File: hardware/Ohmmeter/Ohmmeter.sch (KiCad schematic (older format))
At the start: 52 parts, among them Q1 KT361, Q10 KT361, Q11 KT361, Q2 KT361, Q3 KT361, Q4 KT361, Q5 KT361, Q6 KT361, Q7 KT361, Q8 KT361, Q9 KT361, U1 L78L05_TO92, U2 LP2950-3.3_TO92, U3 ATmega8A-PU

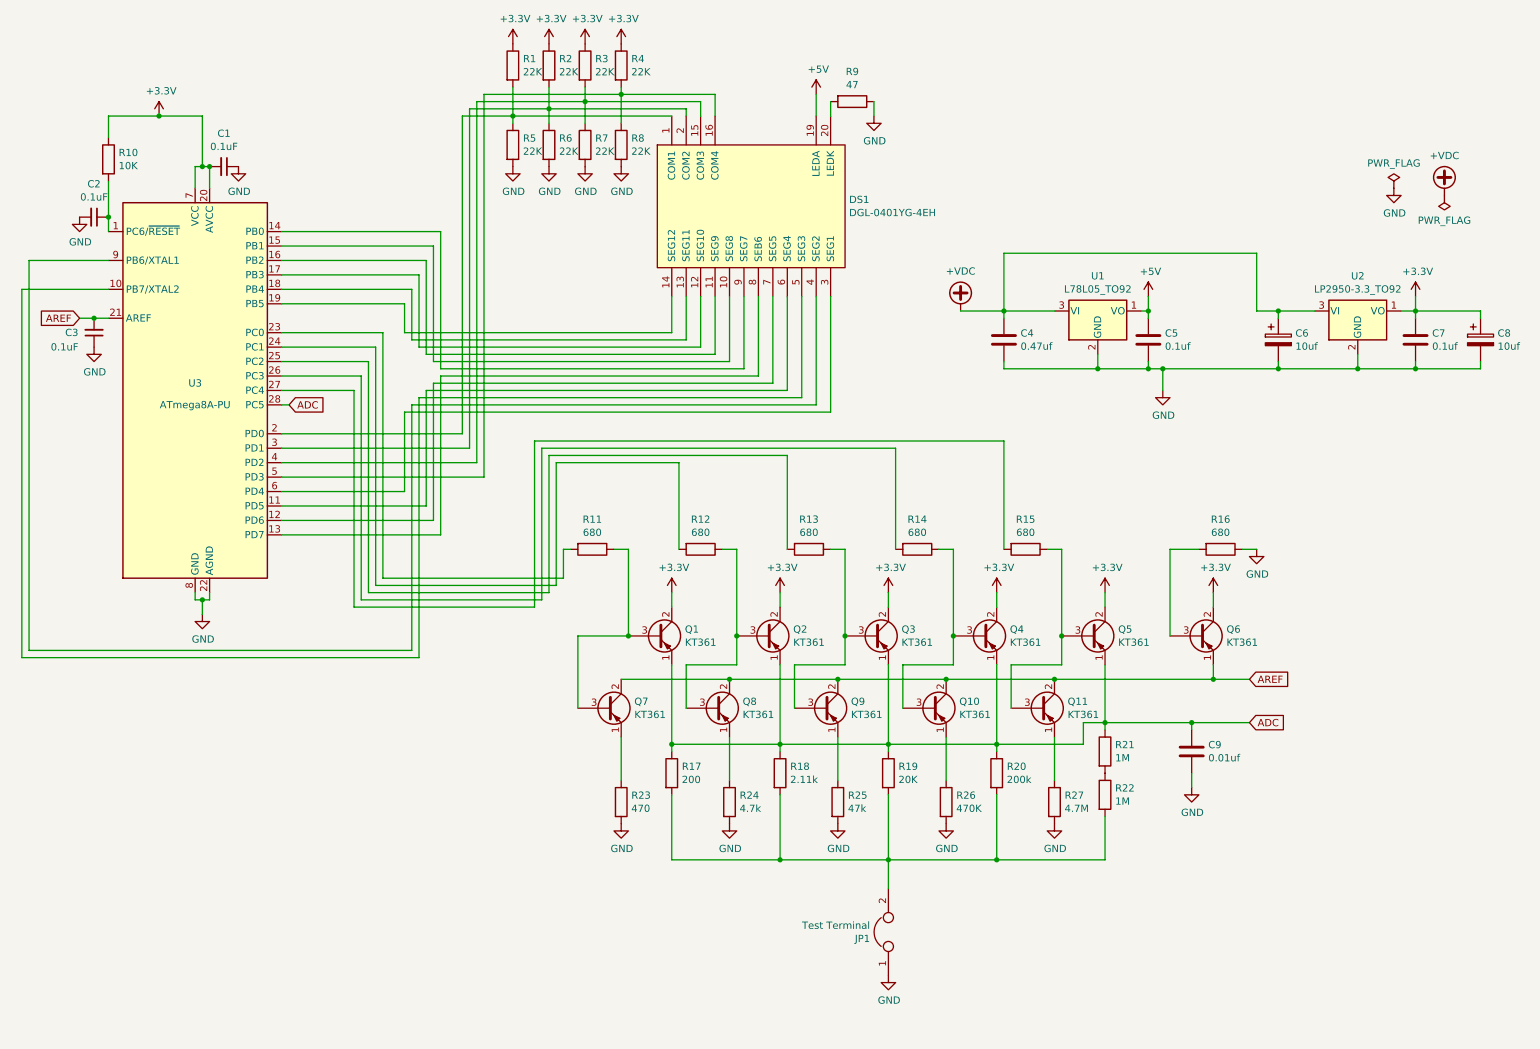
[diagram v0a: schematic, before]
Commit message: Hardware updates. Changed the algorithm to use fewer lookup tables.
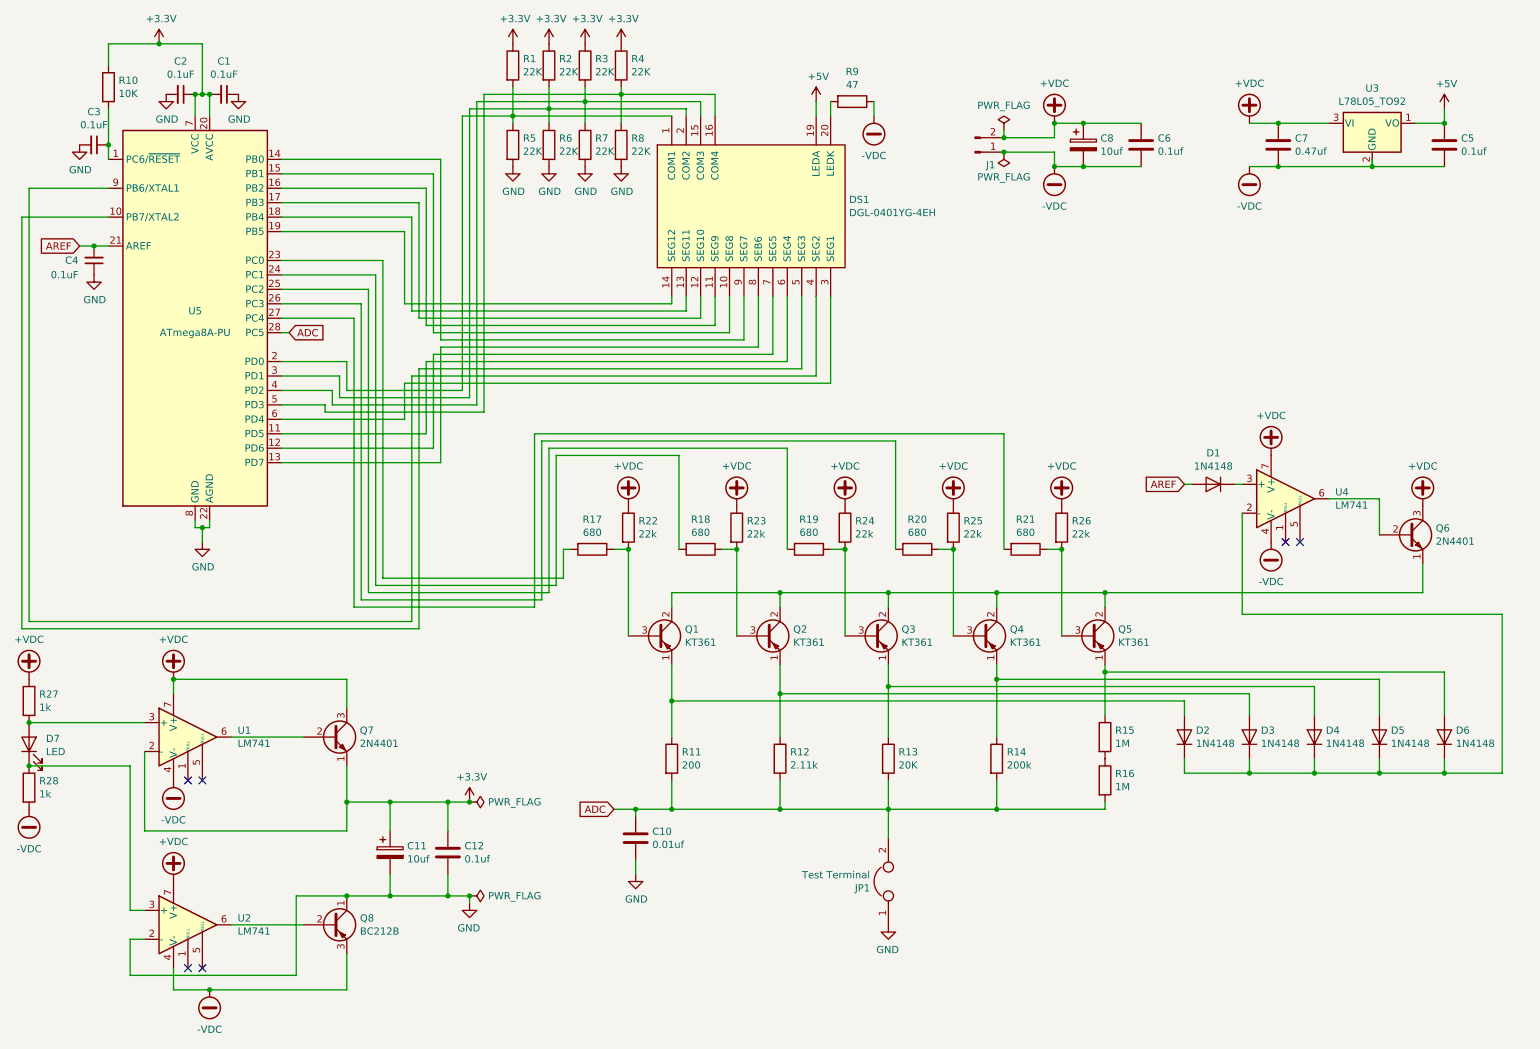
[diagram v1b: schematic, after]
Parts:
- removed C7: 0.1uf, symbol Device:C
- removed C8: 10uf, symbol Device:CP
- removed Q10, Q11, Q6, Q7, Q8, Q9: KT361, symbol Device:Q_PNP_ECB
- removed R16: 680, symbol Device:R
- removed U2: LP2950-3.3_TO92, Package_TO_SOT_THT:TO-92_Inline, symbol Regulator_Linear:LP2950-3.3_TO92
- added C11: 10uf, Capacitor_THT:CP_Radial_D6.3mm_P2.50mm, symbol Device:CP
- added C12, C6: 0.1uf, Resistor_THT:R_Axial_DIN0309_L9.0mm_D3.2mm_P2.54mm_Vertical, symbol Device:C
- added C2: 0.1uF, Resistor_THT:R_Axial_DIN0309_L9.0mm_D3.2mm_P2.54mm_Vertical, symbol Device:C_Small
- added D1, D2, D3, D4, D5, D6: 1N4148, Diode_THT:D_DO-35_SOD27_P7.62mm_Horizontal, symbol Device:D
- added D7: LED, LED_THT:LED_D10.0mm, symbol Device:LED
- added J1: Power, Connector_PinHeader_2.54mm:PinHeader_1x02_P2.54mm_Horizontal, symbol Connector:Conn_01x02_Male
- added Q6, Q7: 2N4401, Package_TO_SOT_THT:TO-92_Inline_Wide, symbol Device:Q_NPN_EBC
- added Q8: BC212B, Package_TO_SOT_THT:TO-92_Inline_Wide, symbol Device:Q_PNP_CBE
- added R22: 22k, Resistor_THT:R_Axial_DIN0207_L6.3mm_D2.5mm_P7.62mm_Horizontal, symbol Device:R
- added R28: 1k, Resistor_THT:R_Axial_DIN0207_L6.3mm_D2.5mm_P7.62mm_Horizontal, symbol Device:R
- added U1, U2, U4: LM741, Package_DIP:DIP-8_W7.62mm_Socket, symbol Amplifier_Operational:LM741
- C1, C5: footprint (none) -> Resistor_THT:R_Axial_DIN0309_L9.0mm_D3.2mm_P2.54mm_Vertical
- C10: renamed from C9; footprint (none) -> Capacitor_THT:C_Rect_L7.0mm_W2.0mm_P5.00mm
- C3: renamed from C2; footprint (none) -> Resistor_THT:R_Axial_DIN0309_L9.0mm_D3.2mm_P2.54mm_Vertical
- C4: renamed from C3; footprint (none) -> Resistor_THT:R_Axial_DIN0309_L9.0mm_D3.2mm_P2.54mm_Vertical
- C7: renamed from C4; footprint (none) -> Capacitor_THT:C_Rect_L7.0mm_W4.5mm_P5.00mm
- C8: renamed from C6; footprint (none) -> Capacitor_THT:CP_Radial_D6.3mm_P2.50mm
- DS1: footprint (none) -> Connector_PinHeader_2.54mm:PinHeader_1x20_P2.54mm_Horizontal
- JP1: footprint (none) -> Connector_PinHeader_2.54mm:PinHeader_1x02_P2.54mm_Horizontal
- Q1, Q2, Q3, Q4, Q5: footprint (none) -> JRMKiCadLibrary:KT-13
- R1, R10, R2, R3, R4, R5, R6, R7, R8, R9: footprint (none) -> Resistor_THT:R_Axial_DIN0207_L6.3mm_D2.5mm_P7.62mm_Horizontal
- R11: renamed from R17; footprint (none) -> Resistor_THT:R_Axial_DIN0207_L6.3mm_D2.5mm_P10.16mm_Horizontal
- R12: renamed from R18; footprint (none) -> Resistor_THT:R_Axial_DIN0207_L6.3mm_D2.5mm_P10.16mm_Horizontal
- R13: renamed from R19; footprint (none) -> Resistor_THT:R_Axial_DIN0207_L6.3mm_D2.5mm_P10.16mm_Horizontal
- R14: renamed from R20; footprint (none) -> Resistor_THT:R_Axial_DIN0207_L6.3mm_D2.5mm_P10.16mm_Horizontal
- R15: renamed from R21; footprint (none) -> Resistor_THT:R_Axial_DIN0614_L14.3mm_D5.7mm_P5.08mm_Vertical
- R16: renamed from R22; footprint (none) -> Resistor_THT:R_Axial_DIN0614_L14.3mm_D5.7mm_P5.08mm_Vertical
- R17: renamed from R11; footprint (none) -> Resistor_THT:R_Axial_DIN0207_L6.3mm_D2.5mm_P7.62mm_Horizontal
- R18: renamed from R12; footprint (none) -> Resistor_THT:R_Axial_DIN0207_L6.3mm_D2.5mm_P7.62mm_Horizontal
- R19: renamed from R13; footprint (none) -> Resistor_THT:R_Axial_DIN0207_L6.3mm_D2.5mm_P7.62mm_Horizontal
- R20: renamed from R14; footprint (none) -> Resistor_THT:R_Axial_DIN0207_L6.3mm_D2.5mm_P7.62mm_Horizontal
- R21: renamed from R15; footprint (none) -> Resistor_THT:R_Axial_DIN0207_L6.3mm_D2.5mm_P7.62mm_Horizontal
- R23: value 470 -> 22k; footprint (none) -> Resistor_THT:R_Axial_DIN0207_L6.3mm_D2.5mm_P7.62mm_Horizontal
- R24: value 4.7k -> 22k; footprint (none) -> Resistor_THT:R_Axial_DIN0207_L6.3mm_D2.5mm_P7.62mm_Horizontal
- R25: value 47k -> 22k; footprint (none) -> Resistor_THT:R_Axial_DIN0207_L6.3mm_D2.5mm_P7.62mm_Horizontal
- R26: value 470K -> 22k; footprint (none) -> Resistor_THT:R_Axial_DIN0207_L6.3mm_D2.5mm_P7.62mm_Horizontal
- R27: value 4.7M -> 1k; footprint (none) -> Resistor_THT:R_Axial_DIN0207_L6.3mm_D2.5mm_P7.62mm_Horizontal
- U3: renamed from U1; footprint Package_TO_SOT_THT:TO-92_Inline -> Package_TO_SOT_THT:TO-92_Inline_Wide
- U5: renamed from U3; footprint Package_DIP:DIP-28_W7.62mm -> Package_DIP:DIP-28_W7.62mm_Socket
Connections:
- net +3V3: now also C11.1, C12.1, C2.1, Q7.1 (E), U1.2 (-); no longer Q1.2 (C), Q2.2 (C), Q3.2 (C), Q4.2 (C), Q5.2 (C)
- net +VDC: now also R23.1, R24.1, R25.1, R26.1, R27.1, C6.1, J1.2 (Pin_2), Q6.3 (C), Q7.3 (C), R22.1, U1.7 (V+), U2.7 (V+), U4.7 (V+)
- net ADC: now also JP1.2, R11.2, R12.2, R13.2, R14.2, R16.2; no longer Q1.1 (E), Q2.1 (E), Q3.1 (E), Q4.1 (E), Q5.1 (E), R11.1, R12.1, R13.1, R14.1, R15.1
- net AREF: now also D1.2 (A)
- net GND: now also C11.2, C12.2, C2.2, Q8.1 (C), U2.2 (-); no longer C5.2, C7.2, C8.2, R23.2, R24.2, R25.2, R26.2, R27.2, R9.1, U3.2 (GND)
- net at Q5.3 (B), R21.1: now also R26.2
- net at Q2.3 (B), R18.1: now also R23.2
- net at Q3.3 (B), R19.1: now also R24.2
- net at Q4.3 (B), R20.1: now also R25.2
- net at Q1.3 (B), R17.1: now also R22.2
- net at DS1.15 (NC): now also R3.2, R7.1, U5.4 (PD2)
- net at DS1.16 (NC): now also R4.2, R8.1, U5.5 (PD3)
- new net: D6.2 (A), Q5.1 (E), R15.1
- new net: Q1.2 (C), Q2.2 (C), Q3.2 (C), Q4.2 (C), Q5.2 (C), Q6.1 (E)
- new net: D3.2 (A), Q2.1 (E), R12.1
- new net: D4.2 (A), Q3.1 (E), R13.1
- new net: D5.2 (A), Q4.1 (E), R14.1
- new net: D2.2 (A), Q1.1 (E), R11.1
- new net: D7.1 (K), R28.1, U2.3 (+)
- new net: D7.2 (A), R27.2, U1.3 (+)
- new net: Q7.2 (B), U1.6
- new net: Q8.2 (B), U2.6
- new net: Q6.2 (B), U4.6
- new net: D2.1 (K), D3.1 (K), D4.1 (K), D5.1 (K), D6.1 (K), U4.2 (-)
- new net: D1.1 (K), U4.3 (+)
- new net -VDC: C5.2, C6.2, C7.2, C8.2, J1.1 (Pin_1), Q8.3 (E), R28.2, R9.1, U1.4 (V-), U2.4 (V-), U3.2 (GND), U4.4 (V-)
- no-connect marks 0 -> 6
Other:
- moved on the sheet: C1, C10, C3, C4, C5, C7, C8, JP1, R10, R11, R12, R13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

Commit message: PCB Fixes.
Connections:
- net at DS1.15 (NC): now also R3.2, R7.1, U5.4 (PD2)
- net at DS1.16 (NC): now also R4.2, R8.1, U5.5 (PD3)
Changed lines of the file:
@@
 	3700 1350 4050 1350
-Wire Wire Line
-	5450 1200 5450 1350
-Wire Wire Line
-	5350 1250 5350 1350
 Wire Wire Line
 	5250 1300 5250 1350
@@
 F 3 "~" H 4050 1000 50  0001 C CNN
 	1    4050 1000
-	1    0    0    -1
-$EndComp
-$Comp
-L Ohmmeter:DGL-0401YG-4EH DS1
-U 1 1 5E114E28
-P 5700 1100
-F 0 "DS1" H 6378 271 50  0000 L CNN
-F 1 "DGL-0401YG-4EH" H 6378 180 50  0000 L CNN
-F 2 "Connector_PinHeader_2.54mm:PinHeader_1x20_P2.54mm_Horizontal" H 5700 1100 50  0001 C CNN
-F 3 "" H 5700 1100 50  0001 C CNN
-	1    5700 1100
 	1    0    0    -1
 $EndComp
@@
 	1    0    0    1
 $EndComp
+$Comp
+L Ohmmeter:DGL-0401YG-4EH DS1
+U 1 1 5E114E28
+P 5700 1100
+F 0 "DS1" H 6378 271 50  0000 L CNN
+F 1 "DGL-0401YG-4EH" H 6378 180 50  0000 L CNN
+F 2 "Connector_PinHeader_2.54mm:PinHeader_1x20_P2.54mm_Horizontal" H 5700 1100 50  0001 C CNN
+F 3 "" H 5700 1100 50  0001 C CNN
+	1    5700 1100
+	1    0    0    -1
+$EndComp
+Wire Wire Line
+	5350 1250 5350 1350
+Wire Wire Line
+	5450 1200 5450 1350
 $EndSCHEMATC
